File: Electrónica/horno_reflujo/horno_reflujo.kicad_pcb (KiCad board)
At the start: 2 copper layers, 189 x 65.9 mm, 42 parts, among them J1 LevelShifter, J10 ssr1, J11 ssr2, J12 encoder, J13 Max6675_modulo2, J14 Max6675_modulo3, J15 Max6675_modulo4, J2 LevelShifter, J3 Display Oled I2C, J4 Max6675_modulo, J5 ESP01, J6 Alimentación y zc, J7 Relevador a ventilador, J8 resistencia, K1 SANYOU_SRD_Form_C, Q1 2N2222A-TO92, U1 LD1117S33TR_SOT223, U3 74LS14

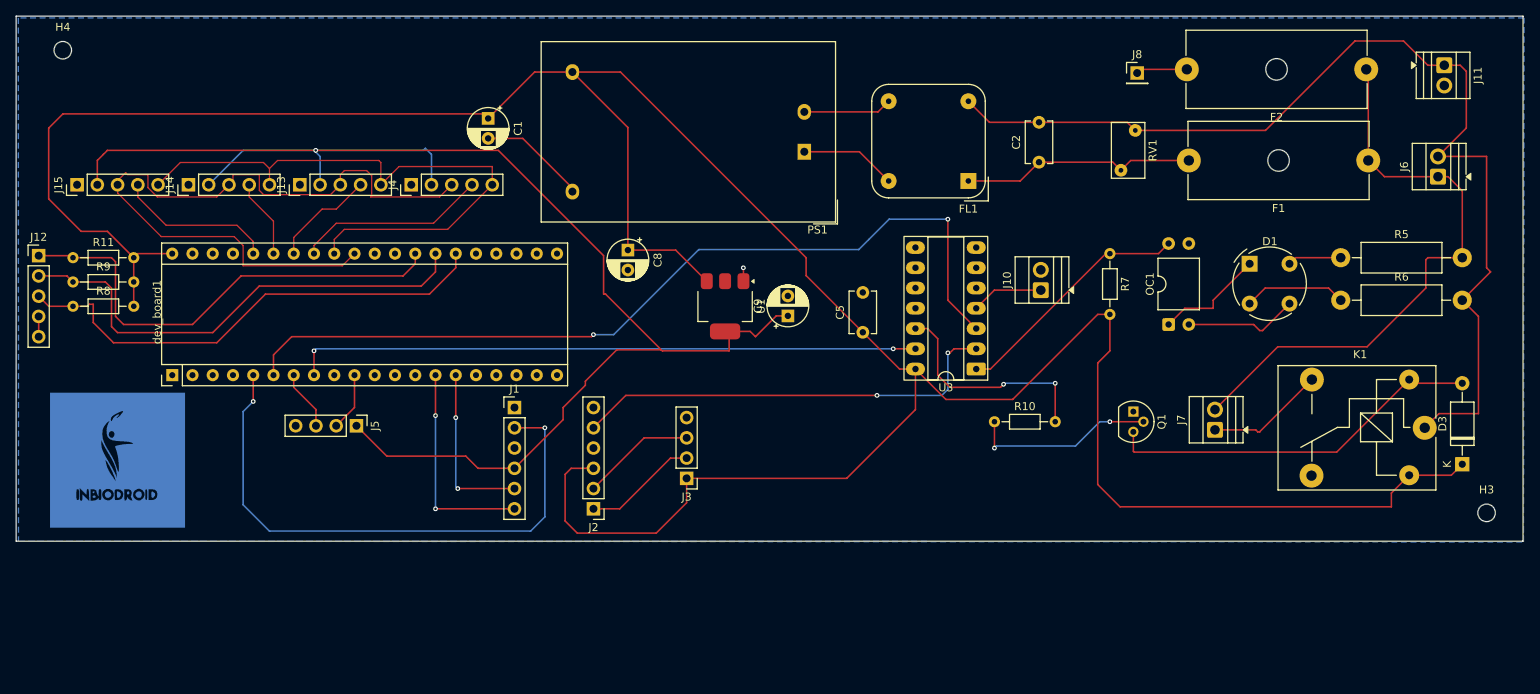
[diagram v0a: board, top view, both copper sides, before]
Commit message: reorganizacion de folders
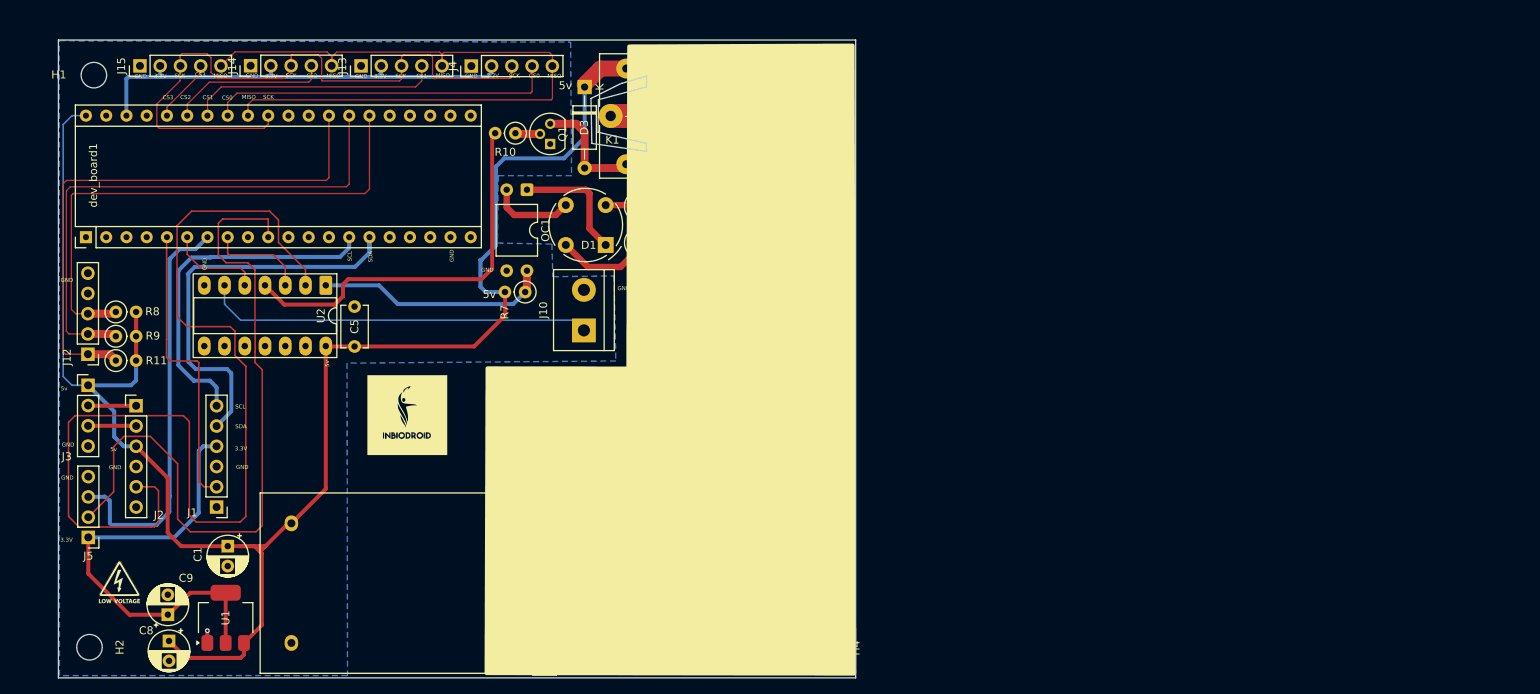
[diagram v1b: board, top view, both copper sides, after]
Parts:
- removed the G*** at (42.4, 79.0)
- removed U3: 74LS14, Package_DIP:DIP-14_W7.62mm_Socket_LongPads
- added G***: LOGO, LOGO, F.Cu at (97.5, 74.9)
- added G***: LOGO, LOGO, F.Cu at (78.8, 73.3)
- added G***: LOGO, LOGO, F.Cu at (42.5, 94.2)
- added H1: MountingHole, MountingHole:MountingHole_3.2mm_M3_DIN965, F.Cu at (39.5, 30.7)
- added H2: MountingHole, MountingHole:MountingHole_3.2mm_M3_DIN965, F.Cu at (38.9, 102.5)
- added U2: 74LS14, Package_DIP:DIP-14_W7.62mm_Socket_LongPads, F.Cu at (68.5, 57.1)
- H3, H4: footprint MountingHole:MountingHole_2.2mm_M2_DIN965 -> MountingHole:MountingHole_3.2mm_M3_DIN965
- J10, J11, J6, J7: footprint TerminalBlock:TerminalBlock_Xinya_XY308-2.54-2P_1x02_P2.54mm_Horizontal -> TerminalBlock:TerminalBlock_bornier-2_P5.08mm
- R10, R11, R7, R8, R9: footprint Resistor_THT:R_Axial_DIN0204_L3.6mm_D1.6mm_P7.62mm_Horizontal -> Resistor_THT:R_Axial_DIN0207_L6.3mm_D2.5mm_P2.54mm_Vertical
- R5, R6: footprint Resistor_THT:R_Axial_DIN0411_L9.9mm_D3.6mm_P15.24mm_Horizontal -> Resistor_THT:R_Axial_DIN0411_L9.9mm_D3.6mm_P5.08mm_Vertical
- moved H4 121.5 mm to (131.2, 102.5), turned to -90 degrees
- moved D3 119.8 mm to (101.0, 32.2), turned to -90 degrees
- moved K1 109.3 mm to (104.3, 35.8), turned to 0 degrees
- moved H3 99.2 mm to (131.8, 30.3), turned to 180 degrees
- moved J6 93.1 mm to (130.9, 95.6)
- moved R6 88.7 mm to (107.9, 47.2)
- moved R5 87.9 mm to (107.9, 51.7)
- moved J11 86.4 mm to (125.5, 52.2), turned to 90 degrees
- moved C9 86.3 mm to (48.7, 98.4)
- moved OC1 82.2 mm to (93.8, 45.1), turned to -90 degrees
- moved D1 80.8 mm to (103.6, 52.0), turned to 180 degrees
- moved Q1 80.5 mm to (96.7, 39.3), turned to 90 degrees
- moved F2 77.6 mm to (133.3, 71.2)
- moved F1 77.2 mm to (133.3, 81.6)
- moved J8 77.2 mm to (104.8, 71.2), turned to 90 degrees
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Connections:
- J13 pad 2: +3.3V -> +3.3Vmc
- J14 pad 2: +3.3V -> +3.3Vmc
- J15 pad 2: +3.3V -> +3.3Vmc
- J4 pad 2: +3.3V -> +3.3Vmc
- J6 pad 1: LINE -> NEUT
- J6 pad 2: NEUT -> LINE
- R5 pad 2: LINE -> Net-(J8-Pin_1)
- dev_board1 pad 38: unconnected-(dev_board1-3.3-Pad38) -> +3.3Vmc
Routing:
- net +5V: track 369.9 -> 219.8 mm
- net +3.3V: track 194.2 -> 57.8 mm, vias 1 -> 0
- net /fire: track 109.4 -> 11.9 mm, vias 2 -> 0
- net LINE: track 74.3 -> 171.3 mm, vias 0 -> 7
- net /Rx_mcu_esp01: track 7.30 -> 89.3 mm
- net zero: track 54.8 -> 133.0 mm, vias 2 -> 0
- net /fan: track 78.6 -> 12.3 mm, vias 2 -> 0
- net +3.3Vmc: track 0.00 -> 58.1 mm
- net NEUT: track 130.7 -> 175.7 mm, vias 0 -> 8
- net /Tx_mcu_esp01: track 7.51 -> 51.9 mm
- net Net-(J10-Pin_1): track 9.04 -> 48.8 mm
- net /zc: track 71.7 -> 38.2 mm, vias 2 -> 0
- net Net-(D3-A): track 47.7 -> 14.7 mm
- net I2C1_SDA: track 21.4 -> 51.7 mm, vias 2 -> 0
- net Net-(J8-Pin_1): track 6.43 -> 28.2 mm
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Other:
- board size 189 x 65.9 mm -> 100 x 80 mm
- board text added: "3.3V"
- board text added: "5v"
- board text added: "CS0"
- board text added: "CS1"
- board text added: "CS2"
- board text added: "CS3"
- board text added: "GND"
- board text added: "LINE VENT"
- board text added: "MISO"
- board text added: "NEUT LINE"
- board text added: "NEUT SSR"
- board text added: "RESISTENCIA"
- board text added: "SCK"
- board text added: "SCL"
- board text added: "SDA"
